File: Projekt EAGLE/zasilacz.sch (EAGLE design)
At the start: 70 parts, among them IC1 7805TV, Q10 2N4126, Q11 2N4126, Q12 2N4126, Q13 2N4126, Q7 2N4126, Q9 2N4126, U1 STM32L100C-DISCO, U2 IR2101, U3 IR2101, U4 IR2101

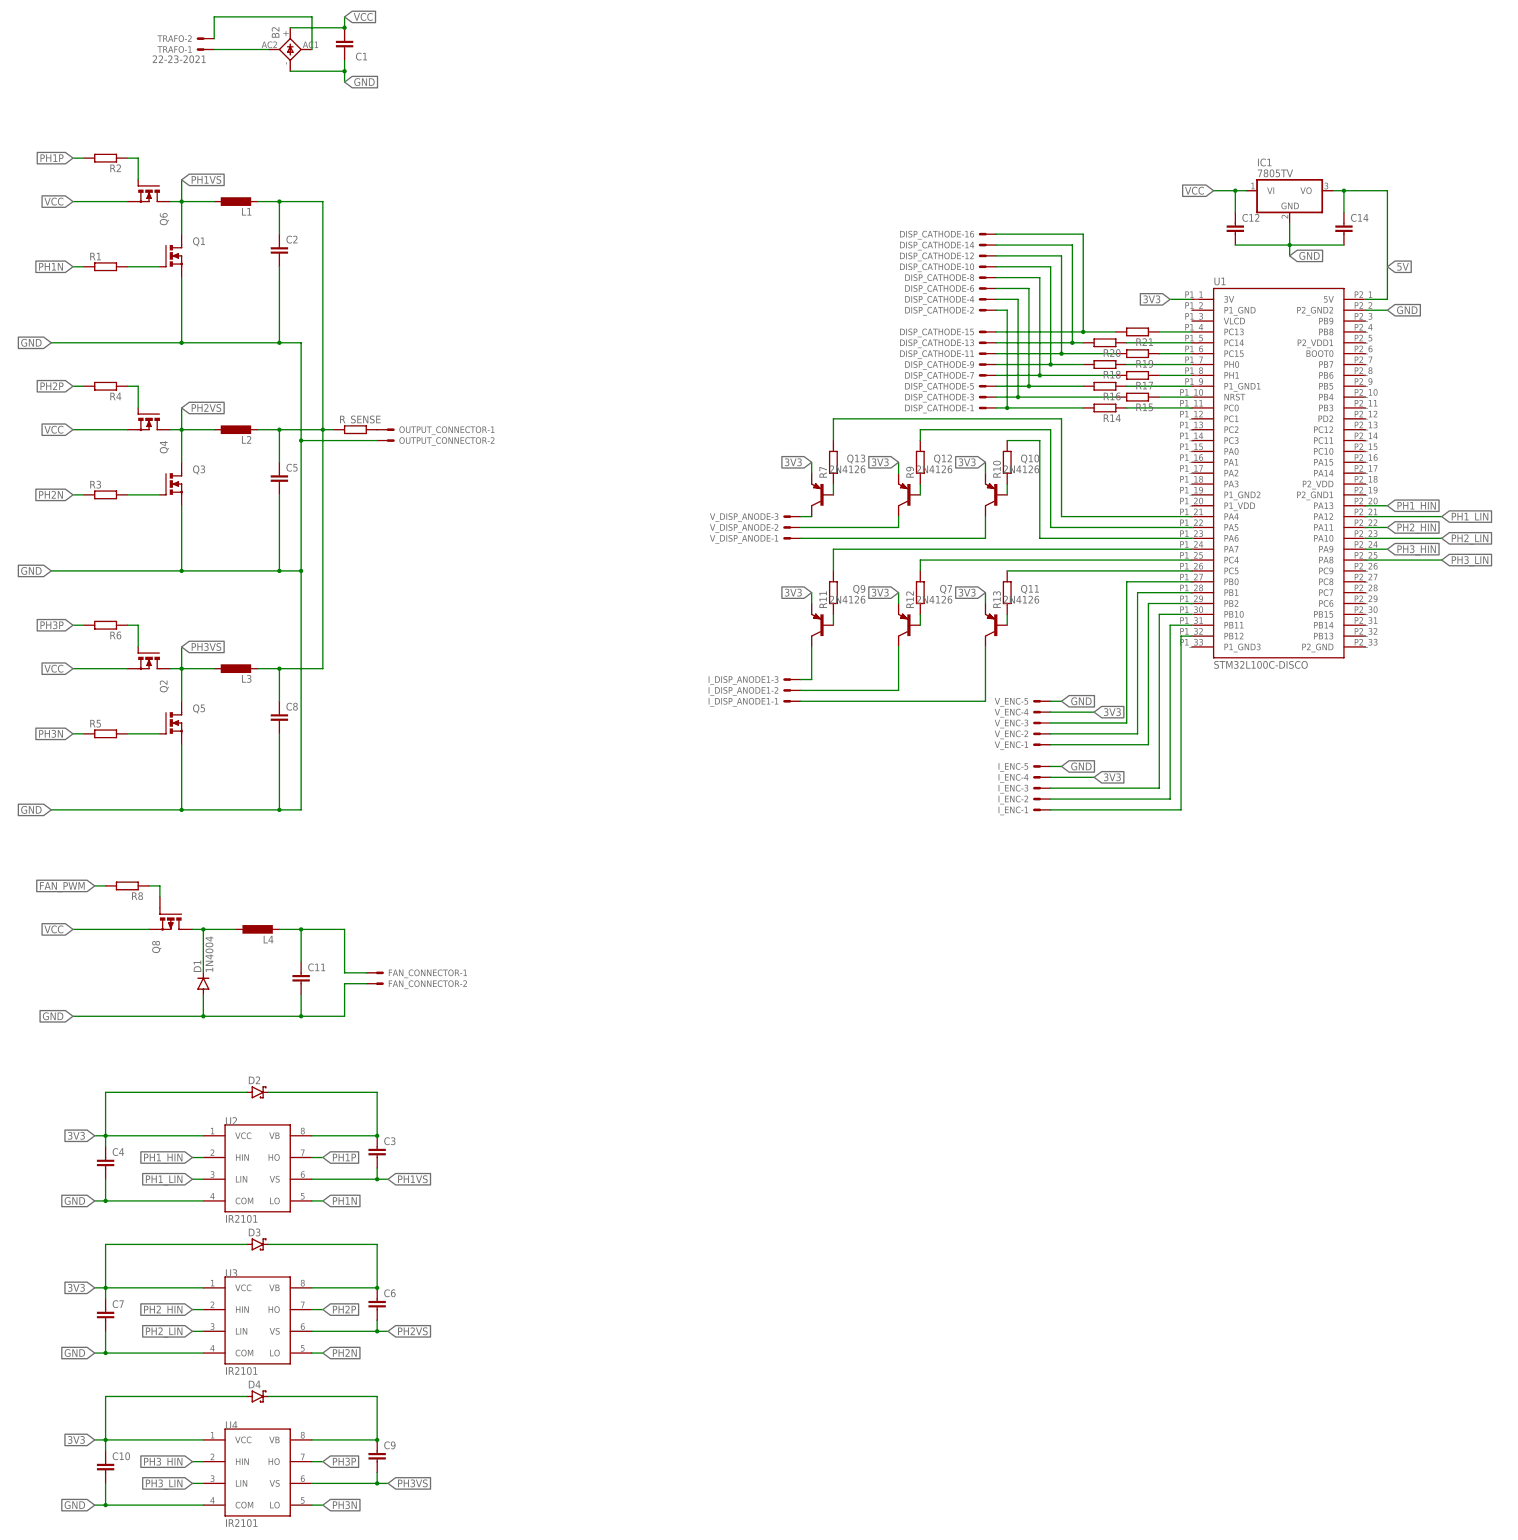
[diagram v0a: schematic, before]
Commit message: .
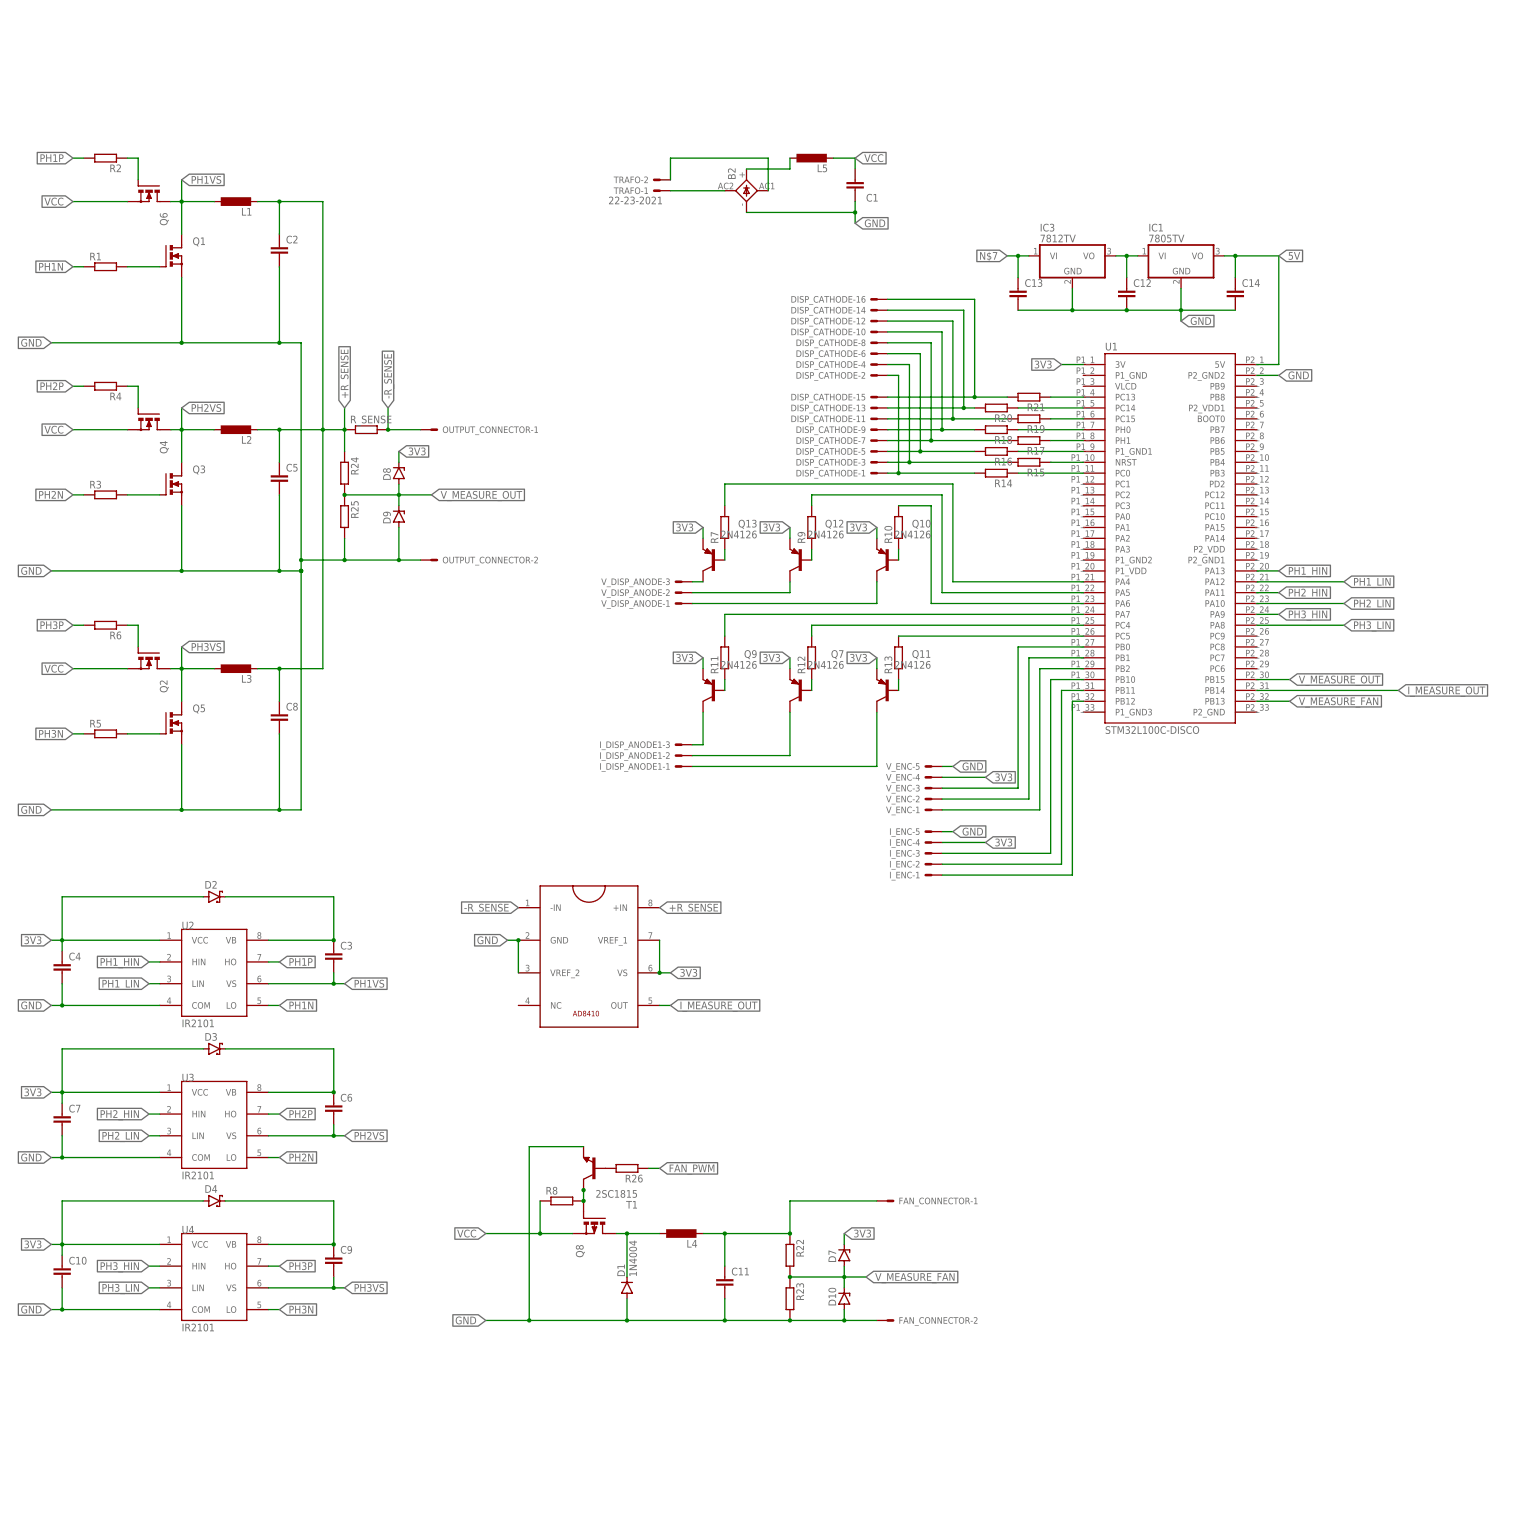
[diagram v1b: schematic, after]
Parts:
- added C13: (no value), rcl:C-EU025-024X044
- added D10, D7, D8, D9: (no value), diode:ZENER-DIODEDO34-7
- added IC3: 7812TV, linear:7812TV
- added L5: (no value), rcl:L-EU0207/10
- added R22, R23, R24, R25, R26: (no value), rcl:R-EU_0309/10
- added T1: 2SC1815, transistor:2SC1815
- added U$1: AD8410AD8410_V1, AD8410:AD8410AD8410_V1
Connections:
- net N$2 renamed -R_SENSE
- removed net N$31: Q8.G, R8.1
- removed net N$34: C11.2, D1.A, FAN_CONNECTOR-2.S
- removed net N$36: C11.1, FAN_CONNECTOR-1.S, L4.2
- removed net PH3OUT+: C2.1, C5.1, C8.1, L1.2, L2.2, L3.2, R_SENSE.1
- removed net PH3OUT-: C2.2, C5.2, C8.2, OUTPUT_CONNECTOR-2.S, Q1.S, Q3.S, Q5.S
- new net +R_SENSE: C2.1, C5.1, C8.1, L1.2, L2.2, L3.2, R24.1, R_SENSE.1
- new net I_MEASURE_OUT: U$1.OUT
- new net N$1: Q8.G, R8.2, T1.C
- new net N$10: U1.PB15
- new net N$12: U1.PB14
- new net N$13: U1.PB13
- new net N$15: D7.C
- new net N$2: R26.2, T1.B
- new net N$6: B2.+, L5.1
- new net N$7: C13.1, IC3.VI
- new net N$9: U$1.VREF_1, U$1.VS
- new net UWY: C11.1, FAN_CONNECTOR-1.S, L4.2, R22.1
- new net V_MEASURE_FAN: D10.C, D7.A, R22.2, R23.1
- new net V_MEASURE_OUT: D8.A, D9.C, R24.2, R25.1
- net 3V3: now also D8.C
- net FAN_PWM: now also R26.1; no longer R8.2
- net GND: now also C11.2, C13.2, C2.2, C5.2, C8.2, D1.A, D10.A, D9.A, FAN_CONNECTOR-2.S, IC3.GND, OUTPUT_CONNECTOR-2.S, Q1.S, Q3.S, Q5.S, R23.2, R25.2, T1.E, U$1.GND, U$1.VREF_2
- net VCC: now also IC3.VO, L5.2, R8.1; no longer B2.+
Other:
- moved on the sheet: B2, C1, C10, C11, C12, C14, C3, C4, C6, C7, C9, D1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
